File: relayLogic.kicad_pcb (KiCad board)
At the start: 2 copper layers, 33 x 25.4 mm, 5 parts, among them J1 Conn_01x08, J2 Conn_01x08, K1 Relay_DPDT

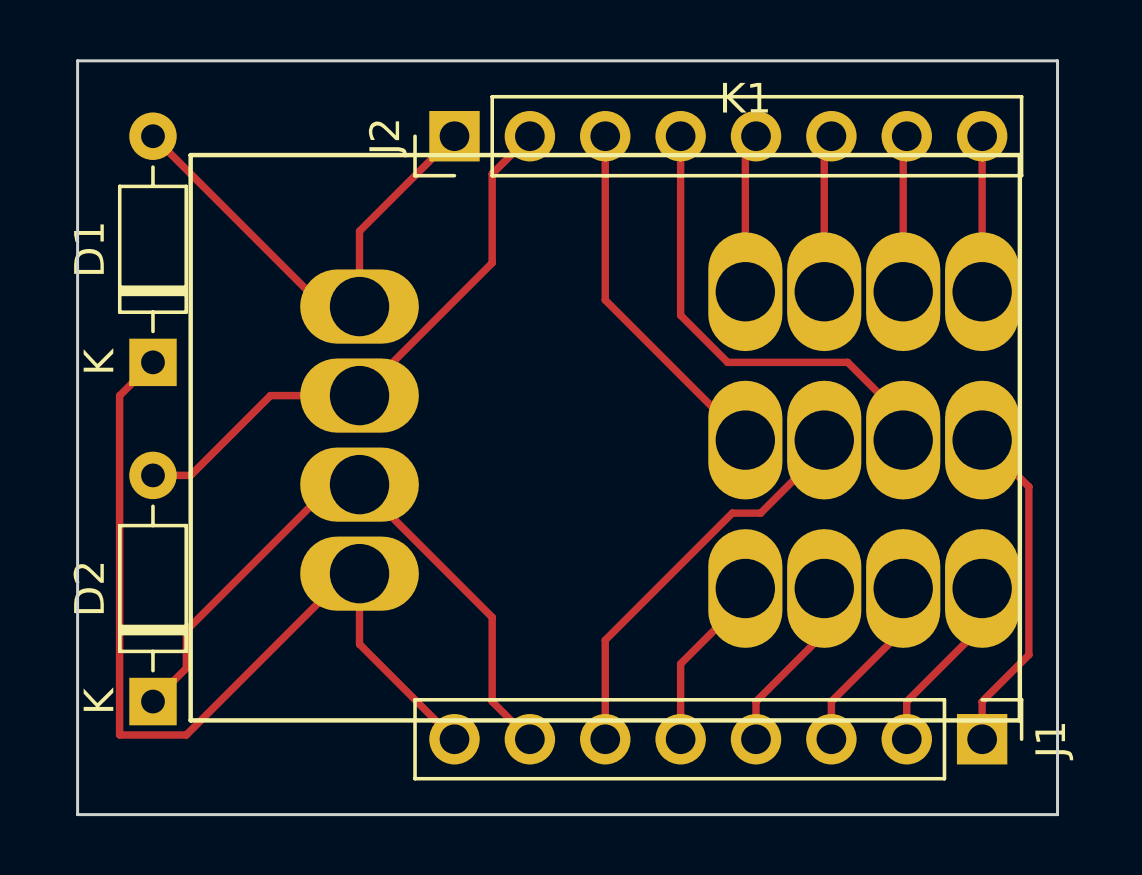
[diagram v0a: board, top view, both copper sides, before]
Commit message: update
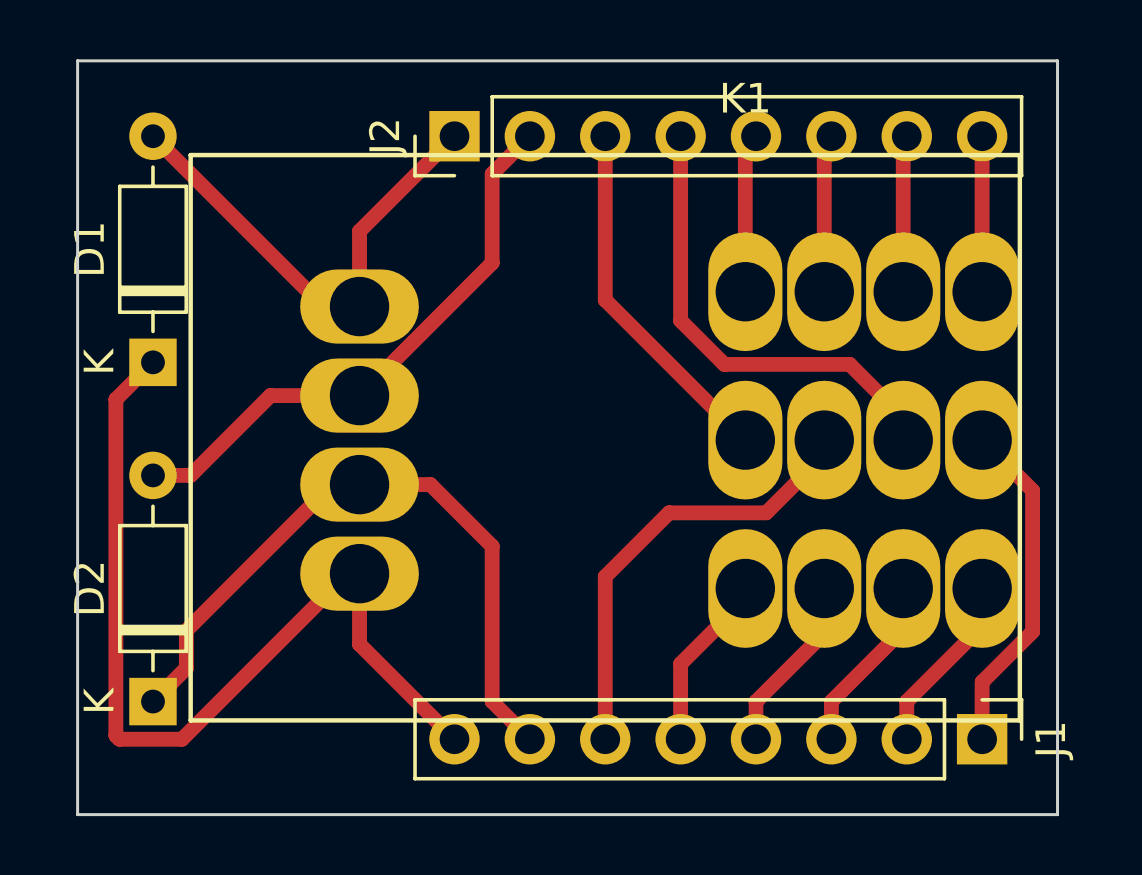
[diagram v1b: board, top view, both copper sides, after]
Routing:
- net Net-(D2-K): track 21.7 -> 23.1 mm
- net Net-(J1-Pin_6): track 13.7 -> 15.1 mm
